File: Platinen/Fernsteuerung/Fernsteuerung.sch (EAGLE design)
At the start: 4 parts, among them K1 ESP32DEVKITV11000MIL, P1 TFT_3.5"_SPI_480X320, U1 COM-09032

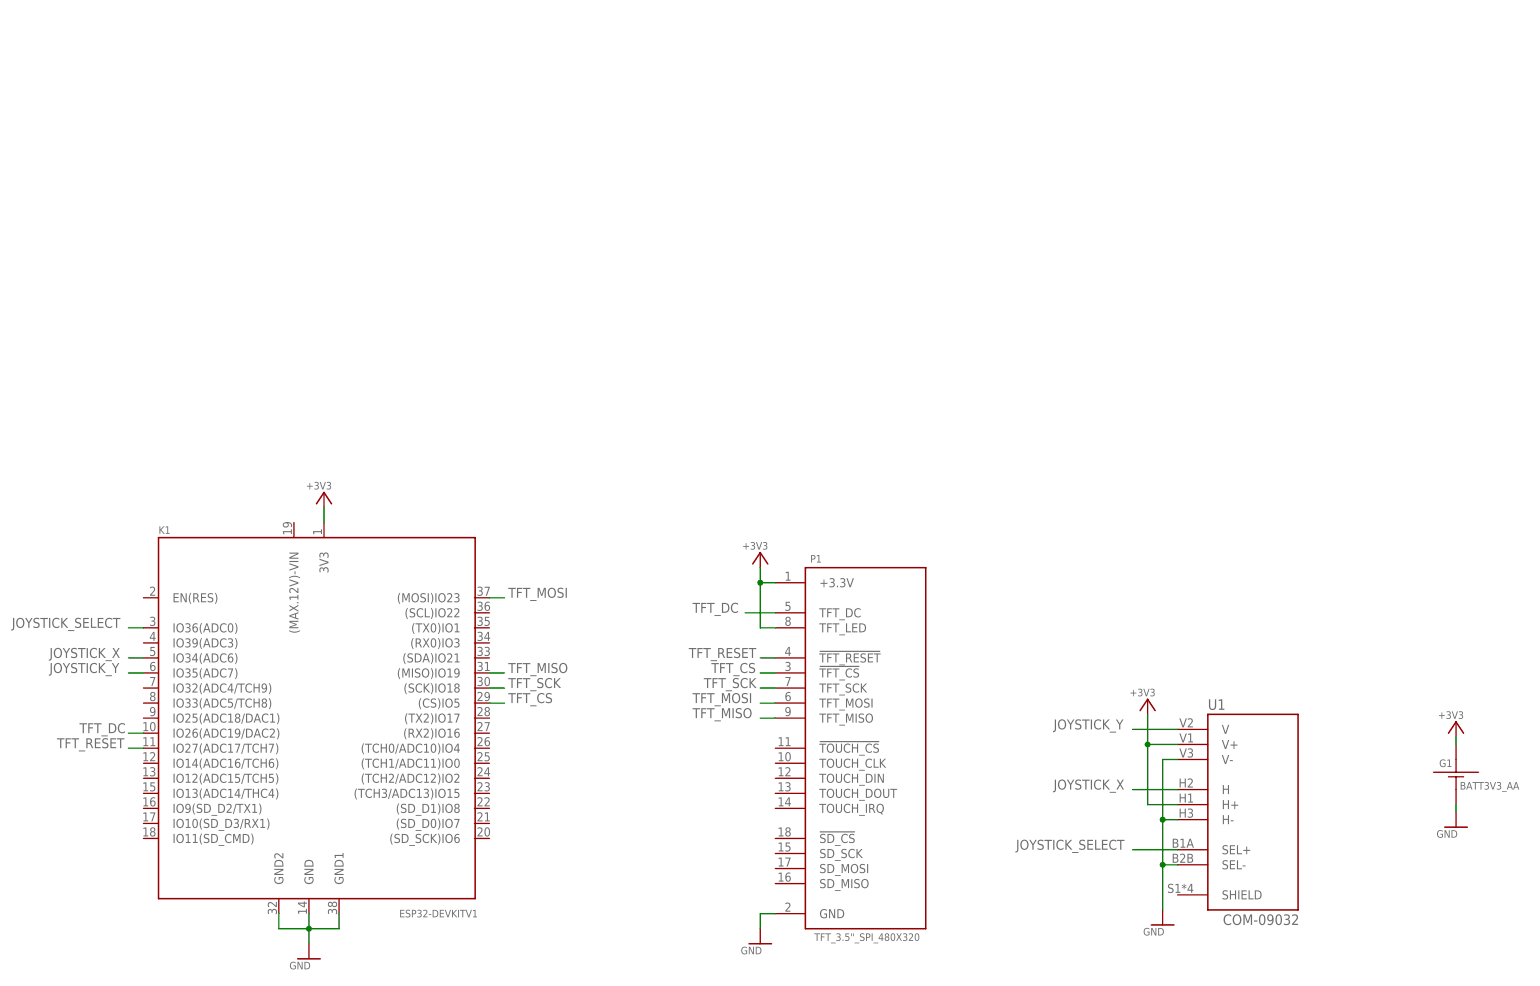
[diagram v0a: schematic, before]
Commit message: board fersteuerung
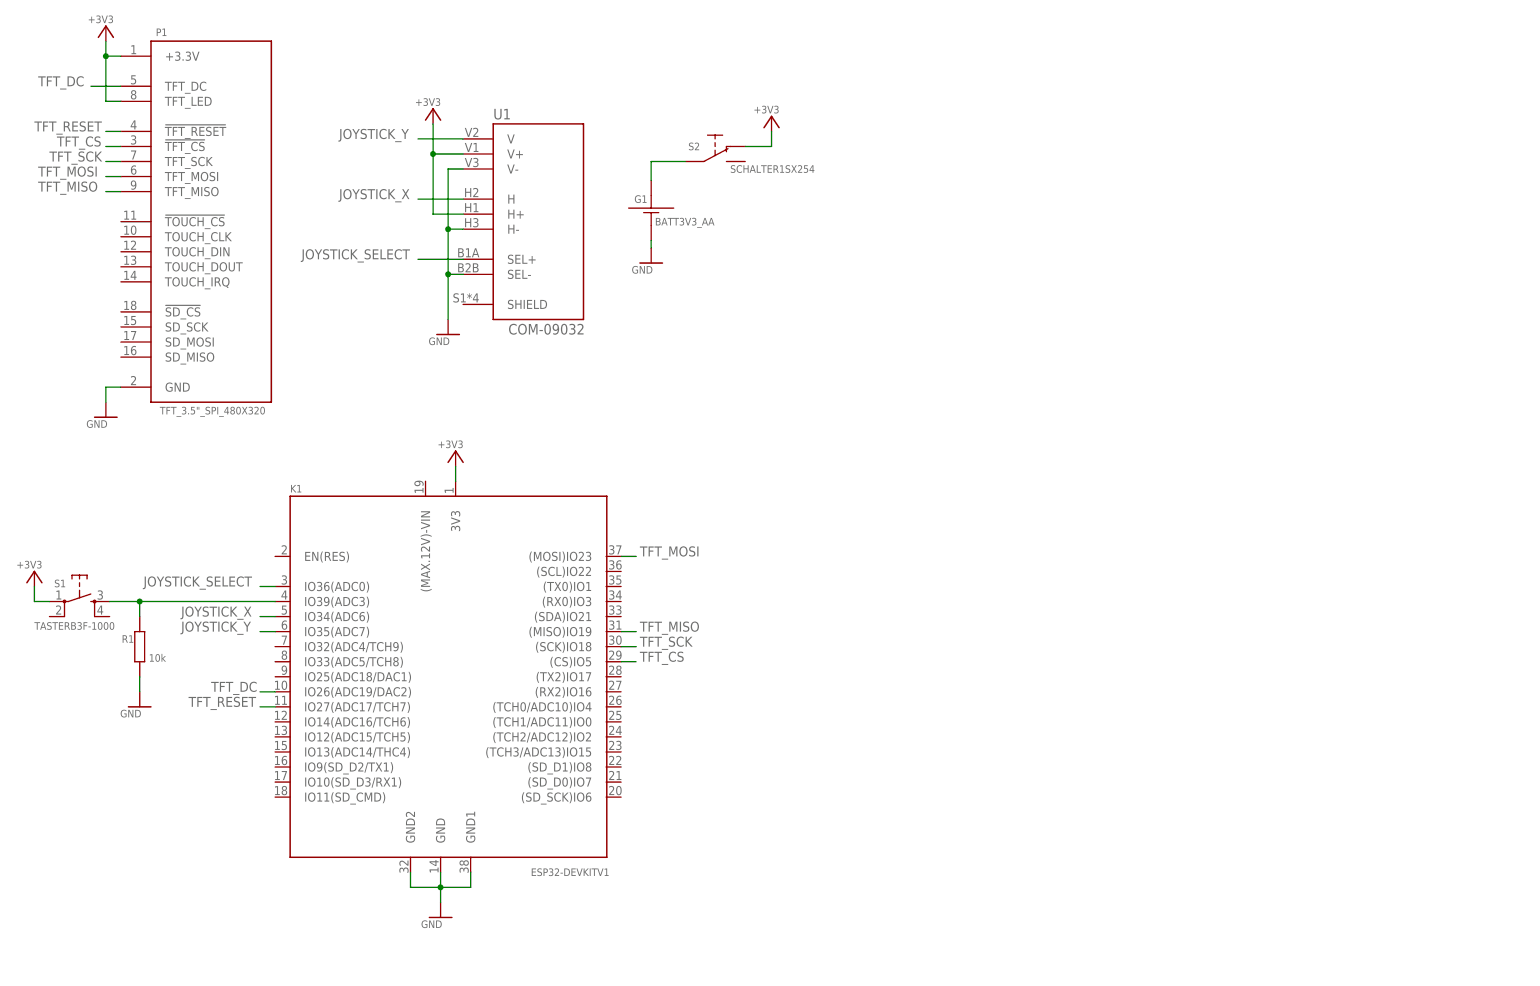
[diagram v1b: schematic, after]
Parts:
- added R1: 10k, HTL22_basis:R1206
- added S1: TASTERB3F-1000, HTL22_basis:TASTERB3F-1000
- added S2: SCHALTER1SX254, HTL22_basis:SCHALTER1SX254
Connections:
- new net N$1: K1.IO39(ADC3), R1.2, S1.S
- new net N$2: G1.PLUS, S2.W1
- net +3V3: now also S1.P, S2.O1; no longer G1.PLUS
- net GND: now also R1.1
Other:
- moved on the sheet: G1, K1, P1, U1
